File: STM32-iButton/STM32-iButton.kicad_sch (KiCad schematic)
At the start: 12 parts, among them J1 Conn_SWD, J2 Conn_SWD, P1 USB_C_2.0, SW1 Button_user, SW2 Button_user, SW3 Button_user, U1 STM32L052C8Tx, U2 AMS1117-3.3

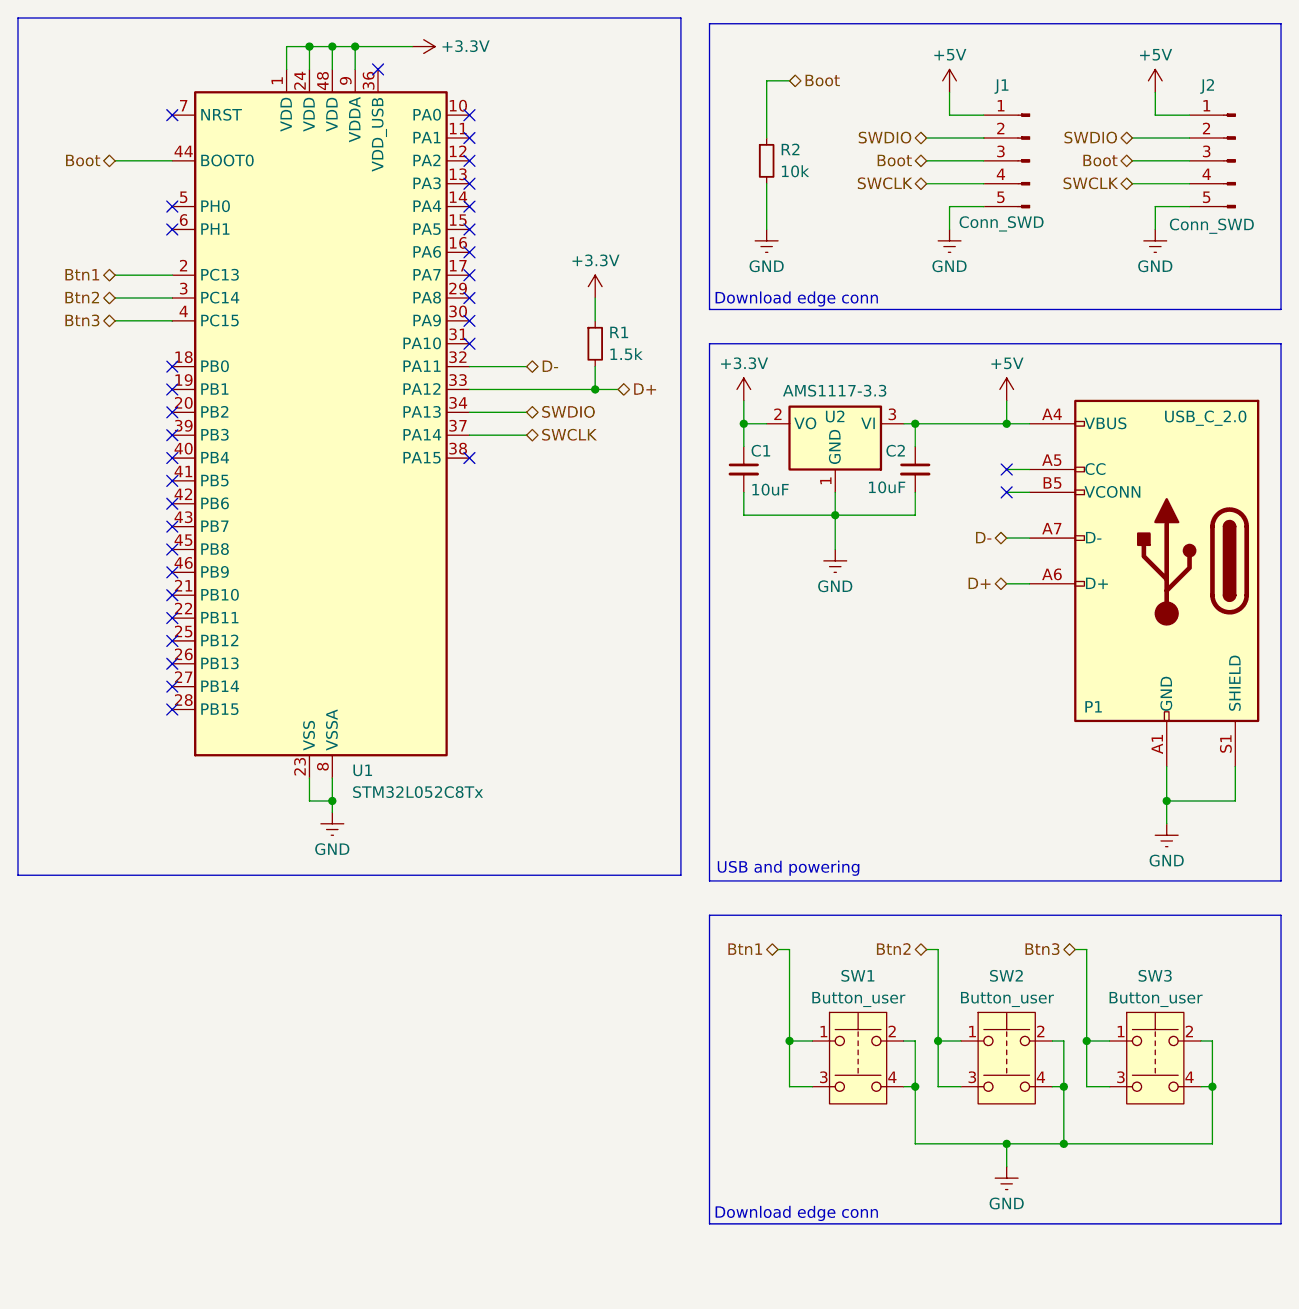
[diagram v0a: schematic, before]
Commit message: updated
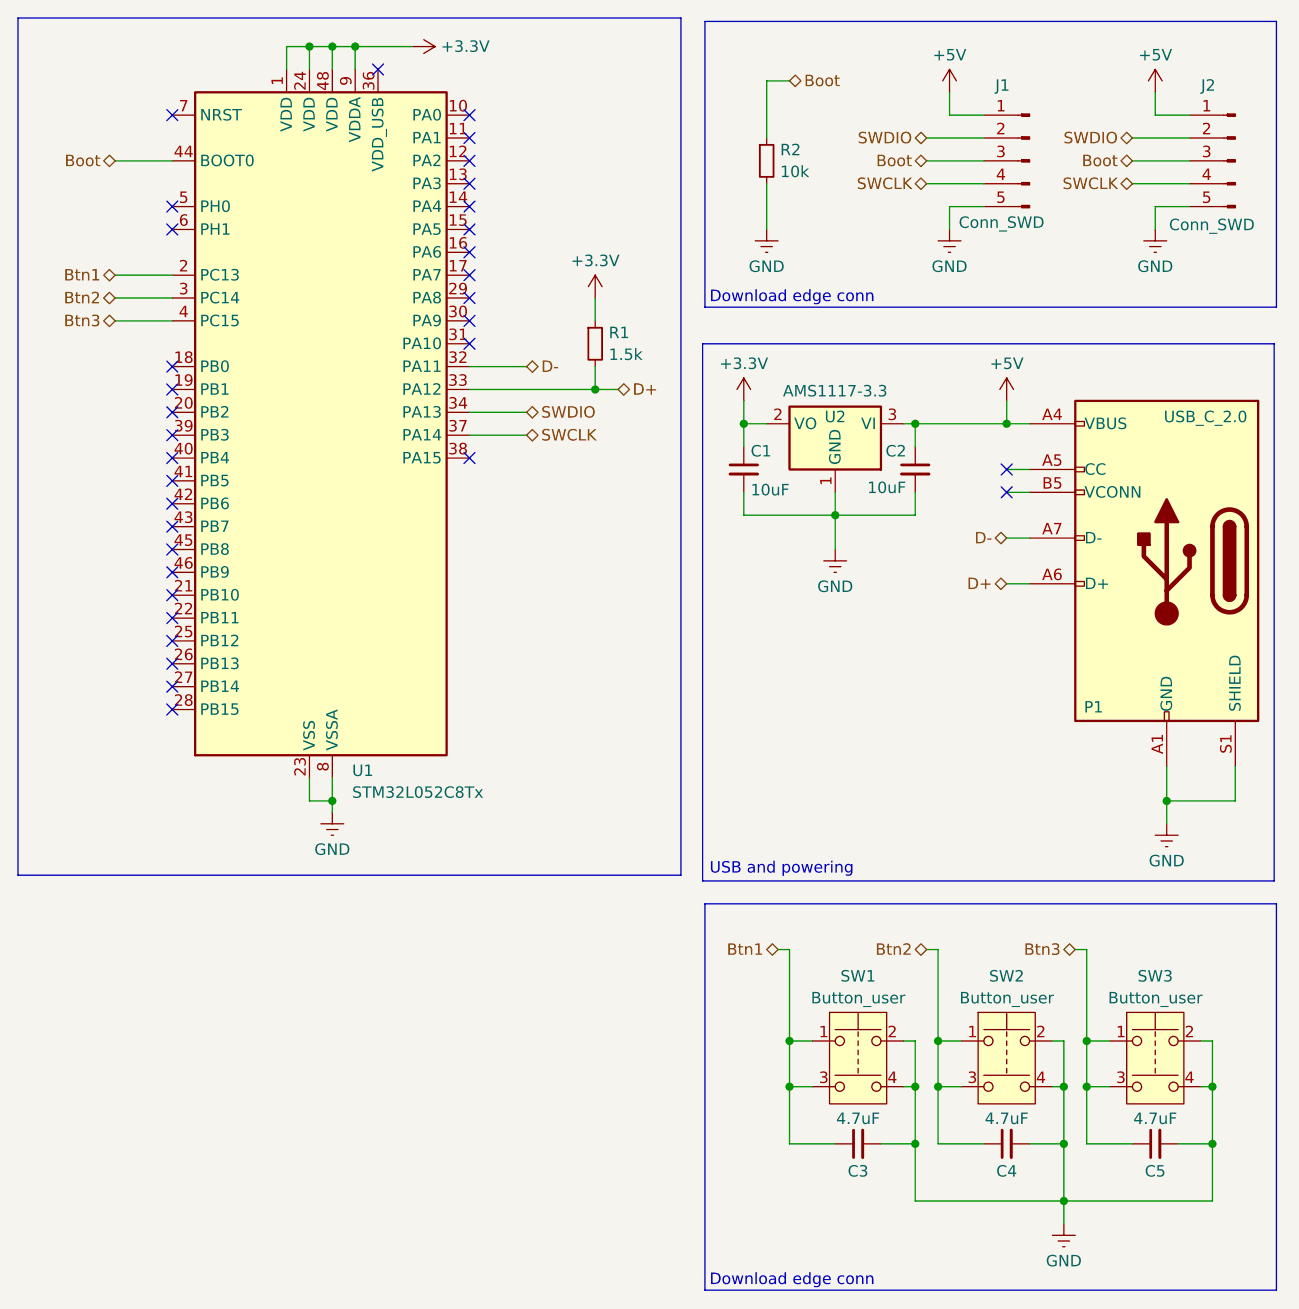
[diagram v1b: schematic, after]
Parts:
- added C3, C4, C5: 4.7uF, Capacitor_SMD:C_0603_1608Metric_Pad1.08x0.95mm_HandSolder, symbol Device:C_Small
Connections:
- net Btn1: now also C3.1
- net Btn2: now also C4.1
- net Btn3: now also C5.1
- net GND: now also C3.2, C4.2, C5.2
